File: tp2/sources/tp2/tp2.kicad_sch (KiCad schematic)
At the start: 21 parts, among them Q1 NPN, U2 ${SIM.PARAMS}, U3 ${SIM.PARAMS}, U4 ${SIM.PARAMS}, U5 ${SIM.PARAMS}, U6 ${SIM.PARAMS}

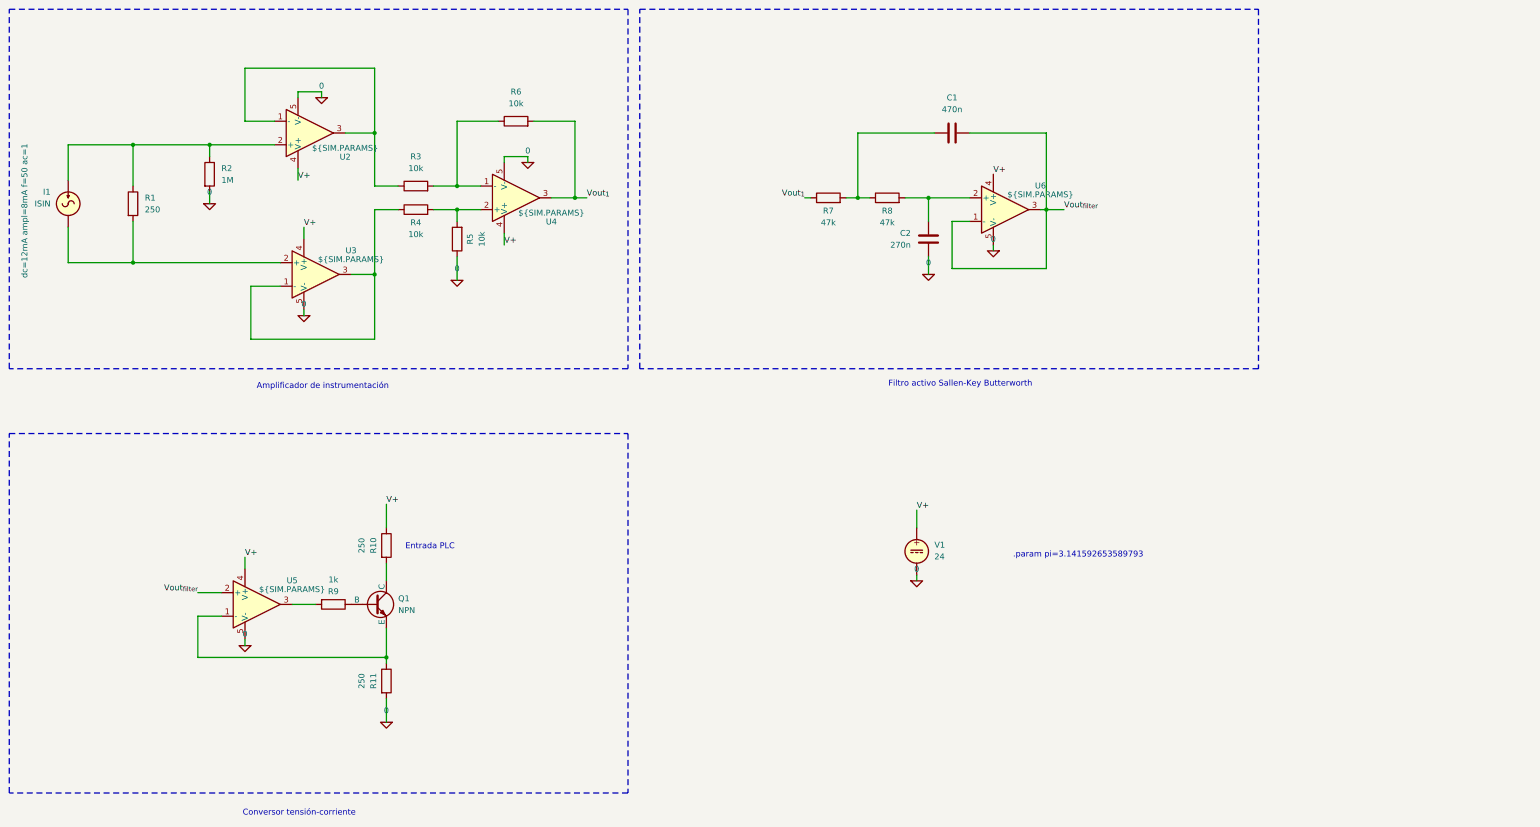
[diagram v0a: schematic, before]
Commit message: tp2: agrega pcb
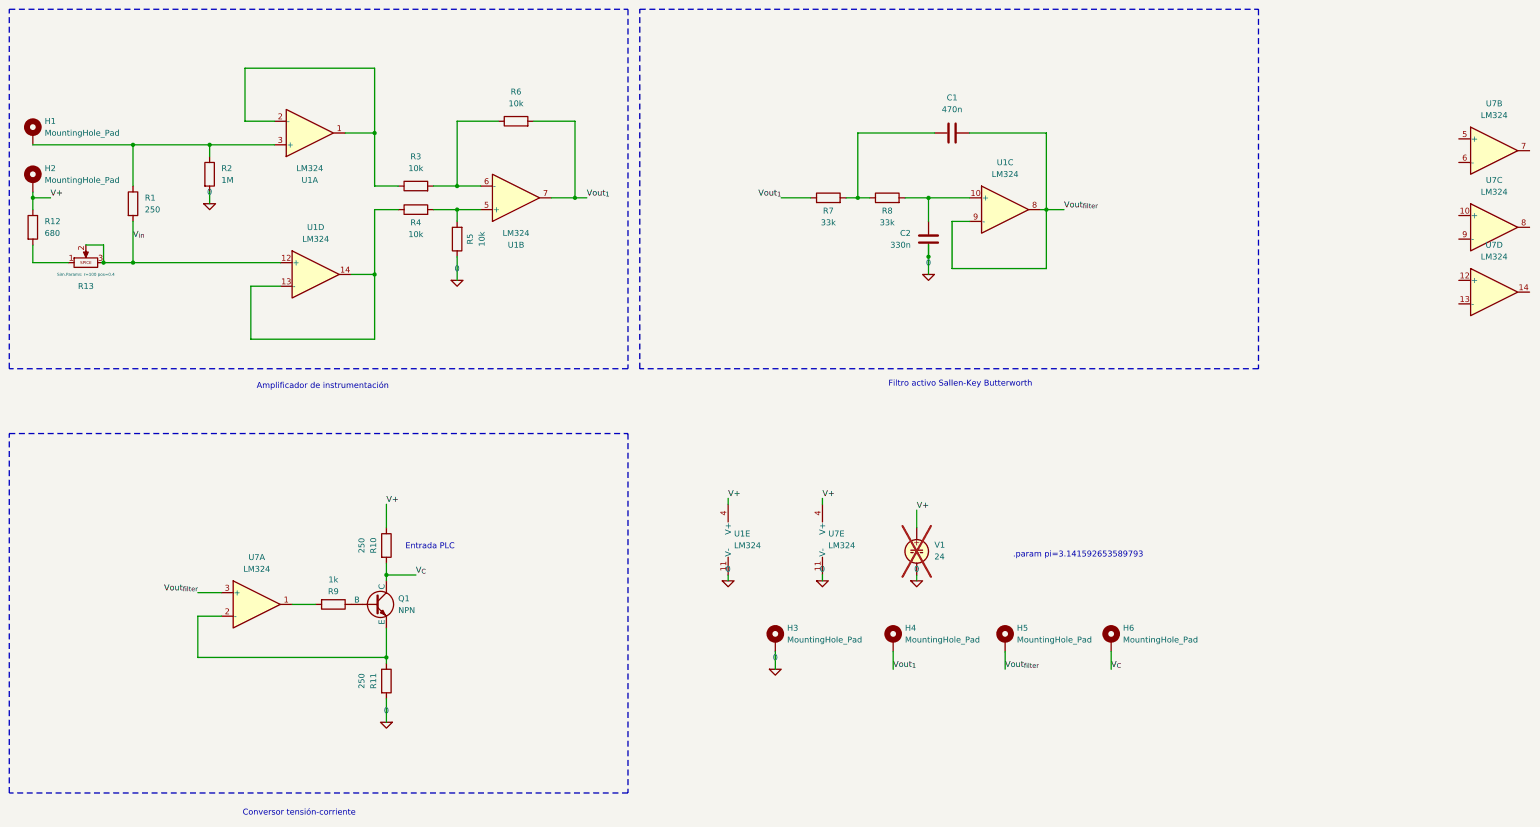
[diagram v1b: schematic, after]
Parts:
- removed I1: ISIN, symbol Simulation_SPICE:ISIN
- removed U2, U3, U4, U5, U6: ${SIM.PARAMS}, symbol Simulation_SPICE:OPAMP
- added H1, H2, H3, H4, H5, H6: MountingHole_Pad, TestPoint:TestPoint_THTPad_2.0x2.0mm_Drill1.0mm, symbol Mechanical:MountingHole_Pad
- added R12: 680, Resistor_THT:R_Axial_DIN0207_L6.3mm_D2.5mm_P7.62mm_Horizontal, symbol Device:R
- added R13: Potentiometer, Potentiometer_THT:Potentiometer_Bourns_3266Y_Vertical, symbol Simulation_SPICE:Potentiometer
- added U1, U7: LM324, Package_DIP:DIP-14_W7.62mm_Socket, symbol Amplifier_Operational:LM324
- C1: footprint (none) -> Capacitor_THT:C_Rect_L7.2mm_W2.5mm_P5.00mm
- C2: value 270n -> 330n; footprint (none) -> Capacitor_THT:C_Rect_L7.2mm_W2.5mm_P5.00mm
- Q1: footprint (none) -> Package_TO_SOT_THT:TO-92
- R1, R10, R11, R2, R3, R4, R5, R6, R9: footprint (none) -> Resistor_THT:R_Axial_DIN0207_L6.3mm_D2.5mm_P7.62mm_Horizontal
- R7, R8: value 47k -> 33k; footprint (none) -> Resistor_THT:R_Axial_DIN0207_L6.3mm_D2.5mm_P7.62mm_Horizontal
- V1: now not fitted; now left out of the parts list
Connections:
- net 0: now also H3.1, U1.11 (V-), U7.11 (V-)
- net V+: now also H2.1, R12.1, U1.4 (V+), U7.4 (V+)
- net Vout_{1}: now also H4.1, U1.7
- net Vout_{filter}: now also H5.1, U1.8, U1.9 (-), U7.3 (+)
- net at R1.1, R2.1: now also H1.1, U1.3 (+)
- net V_{in}: now reaches R1.2
- net V_{in}: now also R13.2, R13.3, U1.12 (+)
- net at C2.2, R8.2: now also U1.10 (+)
- net at R3.2, R6.1: now also U1.6 (-)
- net at R4.2, R5.2: now also U1.5 (+)
- net at R3.1: now also U1.1, U1.2 (-)
- net at Q1.3 (E), R11.1: now also U7.2 (-)
- net at R4.1: now also U1.13 (-), U1.14
- net V_{C}: now reaches Q1.1 (C), R10.2
- net V_{C}: now also H6.1
- net at R9.2: now also U7.1
- new net: R12.2, R13.1
